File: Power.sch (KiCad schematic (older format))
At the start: 5 parts

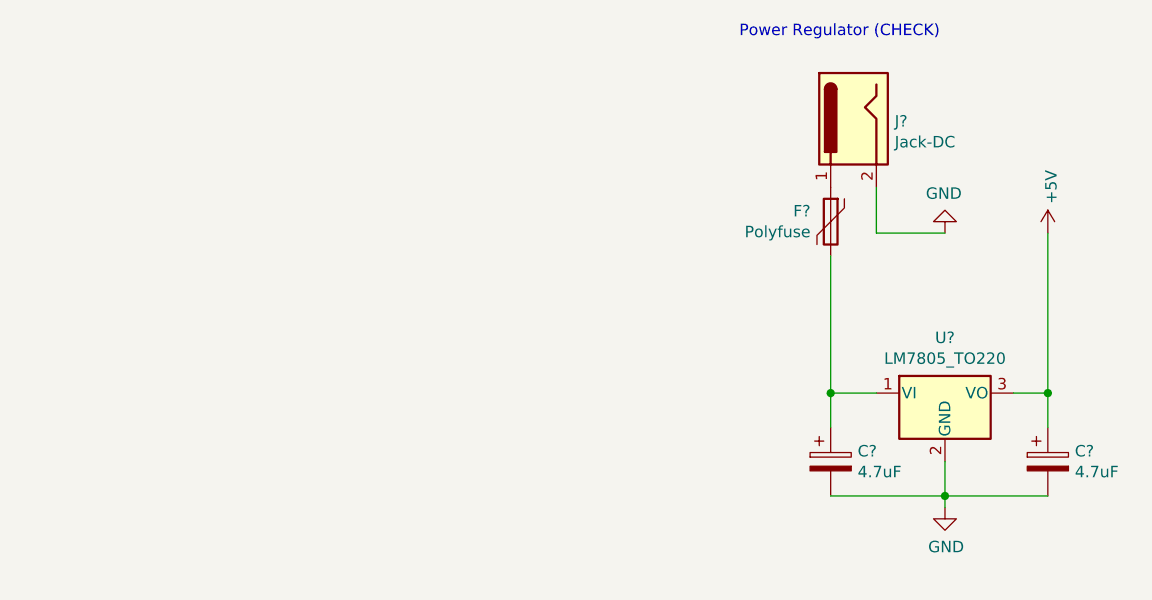
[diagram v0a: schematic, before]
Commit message: more updates
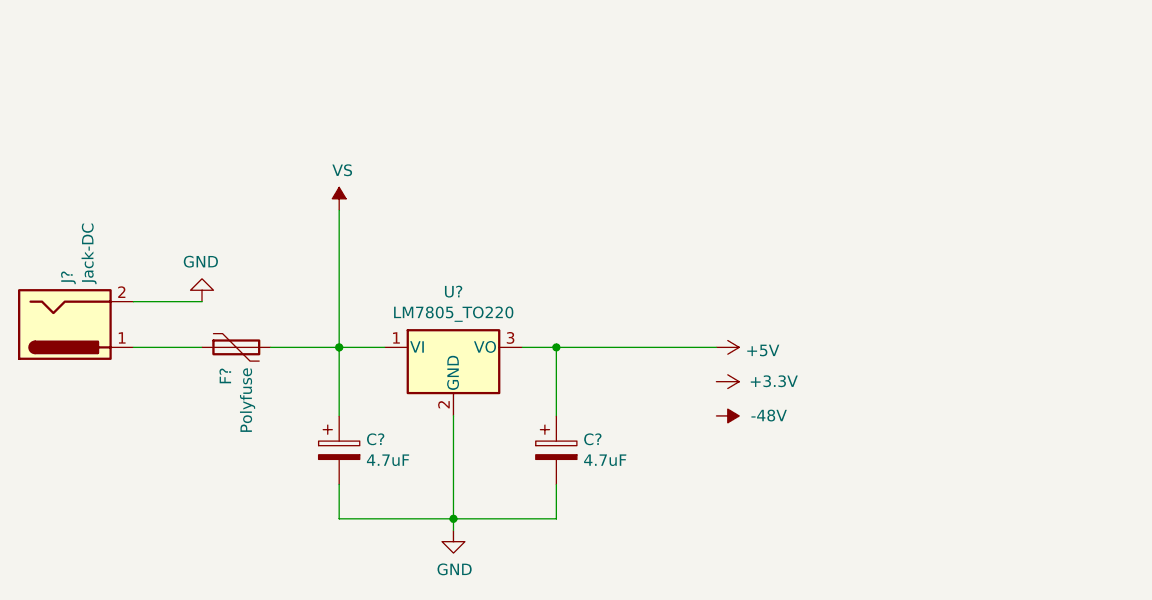
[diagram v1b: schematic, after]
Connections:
- net VS: now reaches C?.1, F?.2, U?.1 (VI)
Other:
- note removed: "Power Regulator (CHECK)"
- moved on the sheet: C?, F?, J?, U?
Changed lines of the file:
@@
 L power:+5V #PWR?
 U 1 1 60E8EED7
-P 6000 3650
+P 4550 4150
 AR Path="/60E8EED7" Ref="#PWR?"  Part="1"
 AR Path="/60E876D5/60E8EED7" Ref="#PWR?"  Part="1"
-F 0 "#PWR?" H 6000 3500 50  0001 C CNN
-F 1 "+5V" V 6015 3778 50  0000 L CNN
-F 2 "" H 6000 3650 50  0001 C CNN
-F 3 "" H 6000 3650 50  0001 C CNN
-	1    6000 3650
-	1    0    0    -1
+F 0 "#PWR?" H 4550 4000 50  0001 C CNN
+F 1 "+5V" V 4565 4278 50  0000 L CNN
+F 2 "" H 4550 4150 50  0001 C CNN
+F 3 "" H 4550 4150 50  0001 C CNN
+	1    4550 4150
+	0    1    1    0
 $EndComp
 $Comp
 L Regulator_Linear:LM7805_TO220 U?
 U 1 1 60E8EEDD
-P 5550 4350
+P 3400 4150
 AR Path="/60E8EEDD" Ref="U?"  Part="1"
 AR Path="/60E876D5/60E8EEDD" Ref="U?"  Part="1"
-F 0 "U?" H 5550 4592 50  0000 C CNN
-F 1 "LM7805_TO220" H 5550 4501 50  0000 C CNN
-F 2 "Package_TO_SOT_THT:TO-220-3_Vertical" H 5550 4575 50  0001 C CIN
-F 3 "https://www.onsemi.cn/PowerSolutions/document/MC7800-D.PDF" H 5550 4300 50  0001 C CNN
-	1    5550 4350
+F 0 "U?" H 3400 4392 50  0000 C CNN
+F 1 "LM7805_TO220" H 3400 4301 50  0000 C CNN
+F 2 "Package_TO_SOT_THT:TO-220-3_Vertical" H 3400 4375 50  0001 C CIN
+F 3 "https://www.onsemi.cn/PowerSolutions/document/MC7800-D.PDF" H 3400 4100 50  0001 C CNN
+	1    3400 4150
 	1    0    0    -1
 $EndComp
@@
 L power:GND #PWR?
 U 1 1 60E8EEE3
-P 5550 4850
+P 3400 4950
 AR Path="/60E8EEE3" Ref="#PWR?"  Part="1"
 AR Path="/60E876D5/60E8EEE3" Ref="#PWR?"  Part="1"
-F 0 "#PWR?" H 5550 4600 50  0001 C CNN
-F 1 "GND" H 5555 4677 50  0000 C CNN
-F 2 "" H 5550 4850 50  0001 C CNN
-F 3 "" H 5550 4850 50  0001 C CNN
-	1    5550 4850
+F 0 "#PWR?" H 3400 4700 50  0001 C CNN
+F 1 "GND" H 3405 4777 50  0000 C CNN
+F 2 "" H 3400 4950 50  0001 C CNN
+F 3 "" H 3400 4950 50  0001 C CNN
+	1    3400 4950
 	1    0    0    -1
 $EndComp
@@
 L Device:C_Polarized C?
 U 1 1 60E8EEE9
-P 5050 4650
+P 2900 4600
 AR Path="/60E8EEE9" Ref="C?"  Part="1"
 AR Path="/60E876D5/60E8EEE9" Ref="C?"  Part="1"
-F 0 "C?" H 5168 4696 50  0000 L CNN
-F 1 "4.7uF" H 5168 4605 50  0000 L CNN
-F 2 "" H 5088 4500 50  0001 C CNN
-F 3 "~" H 5050 4650 50  0001 C CNN
-	1    5050 4650
+F 0 "C?" H 3018 4646 50  0000 L CNN
+F 1 "4.7uF" H 3018 4555 50  0000 L CNN
+F 2 "" H 2938 4450 50  0001 C CNN
+F 3 "~" H 2900 4600 50  0001 C CNN
+	1    2900 4600
 	1    0    0    -1
 $EndComp
@@
 L Device:C_Polarized C?
 U 1 1 60E8EEEF
-P 6000 4650
+P 3850 4600
 AR Path="/60E8EEEF" Ref="C?"  Part="1"
 AR Path="/60E876D5/60E8EEEF" Ref="C?"  Part="1"
-F 0 "C?" H 6118 4696 50  0000 L CNN
-F 1 "4.7uF" H 6118 4605 50  0000 L CNN
-F 2 "" H 6038 4500 50  0001 C CNN
-F 3 "~" H 6000 4650 50  0001 C CNN
-	1    6000 4650
+F 0 "C?" H 3968 4646 50  0000 L CNN
+F 1 "4.7uF" H 3968 4555 50  0000 L CNN
+F 2 "" H 3888 4450 50  0001 C CNN
+F 3 "~" H 3850 4600 50  0001 C CNN
+	1    3850 4600
 	1    0    0    -1
 $EndComp
+Connection ~ 3400 4900
 Wire Wire Line
-	5550 4650 5550 4800
-Connection ~ 5550 4800
+	3400 4900 3400 4950
 Wire Wire Line
-	5550 4800 5550 4850
+	3400 4900 3850 4900
 Wire Wire Line
-	5550 4800 6000 4800
-Wire Wire Line
-	5850 4350 6000 4350
-Wire Wire Line
-	6000 4350 6000 4500
-Text Notes 4650 2800 0    50   ~ 0
-Power Regulator (CHECK)
+	3700 4150 3850 4150
 $Comp
 L Connector:Jack-DC J?
 U 1 1 60E8EEFC
-P 5150 3150
+P 1700 4050
 AR Path="/60E8EEFC" Ref="J?"  Part="1"
 AR Path="/60E876D5/60E8EEFC" Ref="J?"  Part="1"
-F 0 "J?" V 5161 2970 50  0000 R CNN
-F 1 "Jack-DC" V 5252 2970 50  0000 R CNN
-F 2 "" H 5200 3110 50  0001 C CNN
-F 3 "~" H 5200 3110 50  0001 C CNN
-	1    5150 3150
-	0    -1   1    0
+F 0 "J?" V 1711 3870 50  0000 R CNN
+F 1 "Jack-DC" V 1802 3870 50  0000 R CNN
+F 2 "" H 1750 4010 50  0001 C CNN
+F 3 "~" H 1750 4010 50  0001 C CNN
+	1    1700 4050
+	1    0    0    1
 $EndComp
 $Comp
 L power:GND #PWR?
 U 1 1 60E8EF02
-P 5550 3650
+P 2300 3950
 AR Path="/60E8EF02" Ref="#PWR?"  Part="1"
 AR Path="/60E876D5/60E8EF02" Ref="#PWR?"  Part="1"
-F 0 "#PWR?" H 5550 3400 50  0001 C CNN
-F 1 "GND" H 5555 3477 50  0000 C CNN
-F 2 "" H 5550 3650 50  0001 C CNN
-F 3 "" H 5550 3650 50  0001 C CNN
-	1    5550 3650
+F 0 "#PWR?" H 2300 3700 50  0001 C CNN
+F 1 "GND" H 2305 3777 50  0000 C CNN
+F 2 "" H 2300 3950 50  0001 C CNN
+F 3 "" H 2300 3950 50  0001 C CNN
+	1    2300 3950
 	-1   0    0    1
 $EndComp
@@
 L Device:Polyfuse F?
 U 1 1 60E8EF08
-P 5050 3600
+P 2450 4150
 AR Path="/60E8EF08" Ref="F?"  Part="1"
 AR Path="/60E876D5/60E8EF08" Ref="F?"  Part="1"
-F 0 "F?" H 5138 3646 50  0000 L CNN
-F 1 "Polyfuse" H 5138 3555 50  0000 L CNN
-F 2 "" H 5100 3400 50  0001 L CNN
-F 3 "~" H 5050 3600 50  0001 C CNN
-	1    5050 3600
-	-1   0    0    -1
+F 0 "F?" H 2538 4196 50  0000 L CNN
+F 1 "Polyfuse" H 2538 4105 50  0000 L CNN
+F 2 "" H 2500 3950 50  0001 L CNN
+F 3 "~" H 2450 4150 50  0001 C CNN
+	1    2450 4150
+	0    -1   1    0
 $EndComp
 Wire Wire Line
-	5050 3750 5050 4350
+	2900 4900 3400 4900
 Wire Wire Line
-	5050 4800 5550 4800
+	3100 4150 2900 4150
+Connection ~ 2900 4150
 Wire Wire Line
-	5250 4350 5050 4350
-Connection ~ 5050 4350
+	4550 4150 3850 4150
+Connection ~ 3850 4150
 Wire Wire Line
-	5050 4350 5050 4500
+	2300 3950 2000 3950
+$Comp
+L power:+3.3V #PWR?
+U 1 1 60EFCB19
+P 4550 4300
+F 0 "#PWR?" H 4550 4150 50  0001 C CNN
+F 1 "+3.3V" V 4550 4550 50  0000 C CNN
+F 2 "" H 4550 4300 50  0001 C CNN
+F 3 "" H 4550 4300 50  0001 C CNN
+	1    4550 4300
+	0    1    1    0
+$EndComp
 Wire Wire Line
-	6000 3650 6000 4350
-Connection ~ 6000 4350
+	2900 4150 2900 3550
 Wire Wire Line
-	5550 3650 5250 3650
+	2000 4150 2300 4150
 Wire Wire Line
-	5250 3650 5250 3450
+	2600 4150 2900 4150
+Wire Wire Line
+	2900 4150 2900 4450
+Wire Wire Line
+	2900 4750 2900 4900
+Wire Wire Line
+	3400 4450 3400 4900
+Wire Wire Line
+	3850 4750 3850 4900
+Wire Wire Line
+	3850 4150 3850 4450
+$Comp
+L power:-48V #PWR?
+U 1 1 60F10C93
+P 4550 4450
+F 0 "#PWR?" H 4550 4550 50  0001 C CNN
+F 1 "-48V" V 4550 4600 50  0000 L CNN
+F 2 "" H 4550 4450 50  0001 C CNN
+F 3 "" H 4550 4450 50  0001 C CNN
+	1    4550 4450
+	0    1    1    0
+$EndComp
+$Comp
+L power:VS #PWR?
+U 1 1 60F1ACBA
+P 2900 3550
+F 0 "#PWR?" H 2700 3400 50  0001 C CNN
+F 1 "VS" H 2915 3723 50  0000 C CNN
+F 2 "" H 2900 3550 50  0001 C CNN
+F 3 "" H 2900 3550 50  0001 C CNN
+	1    2900 3550
+	1    0    0    -1
+$EndComp
 $EndSCHEMATC
